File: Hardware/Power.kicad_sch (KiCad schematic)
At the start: 62 parts

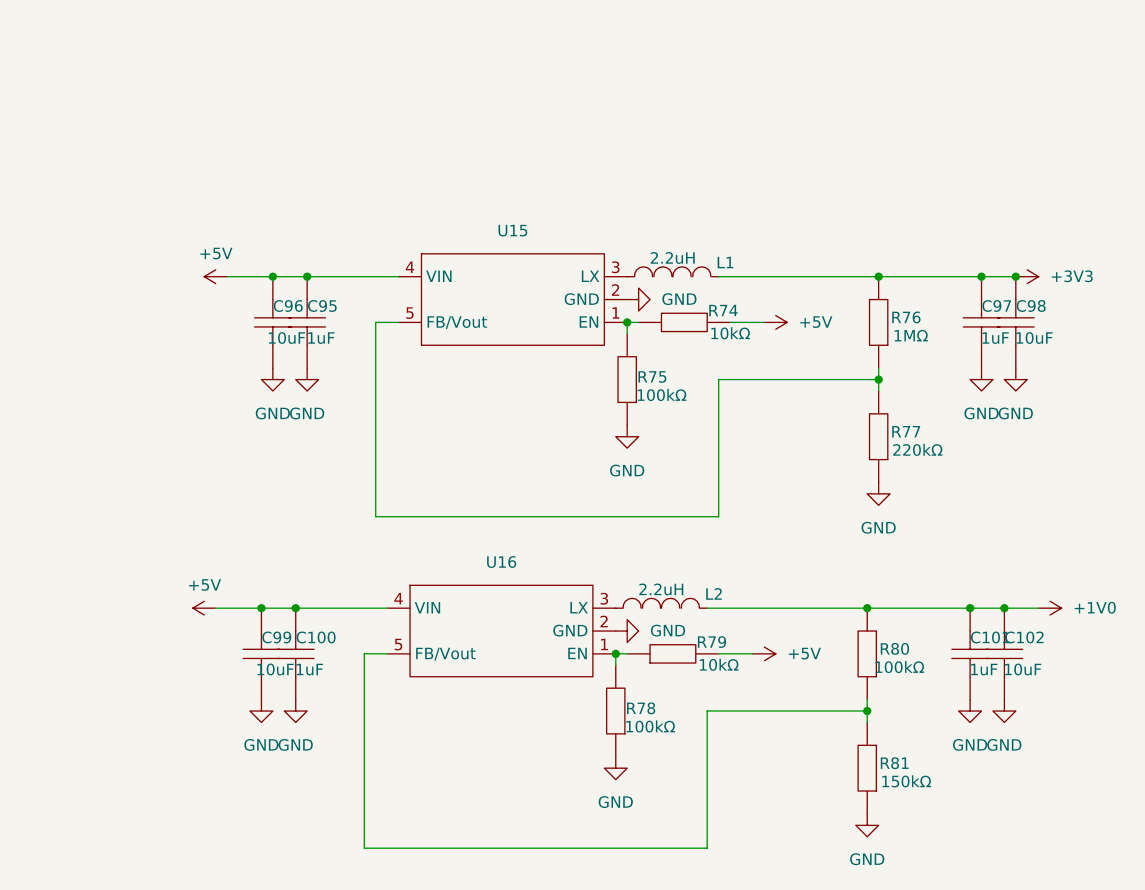
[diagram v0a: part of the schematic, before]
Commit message: 修改了电源供电部分的内容
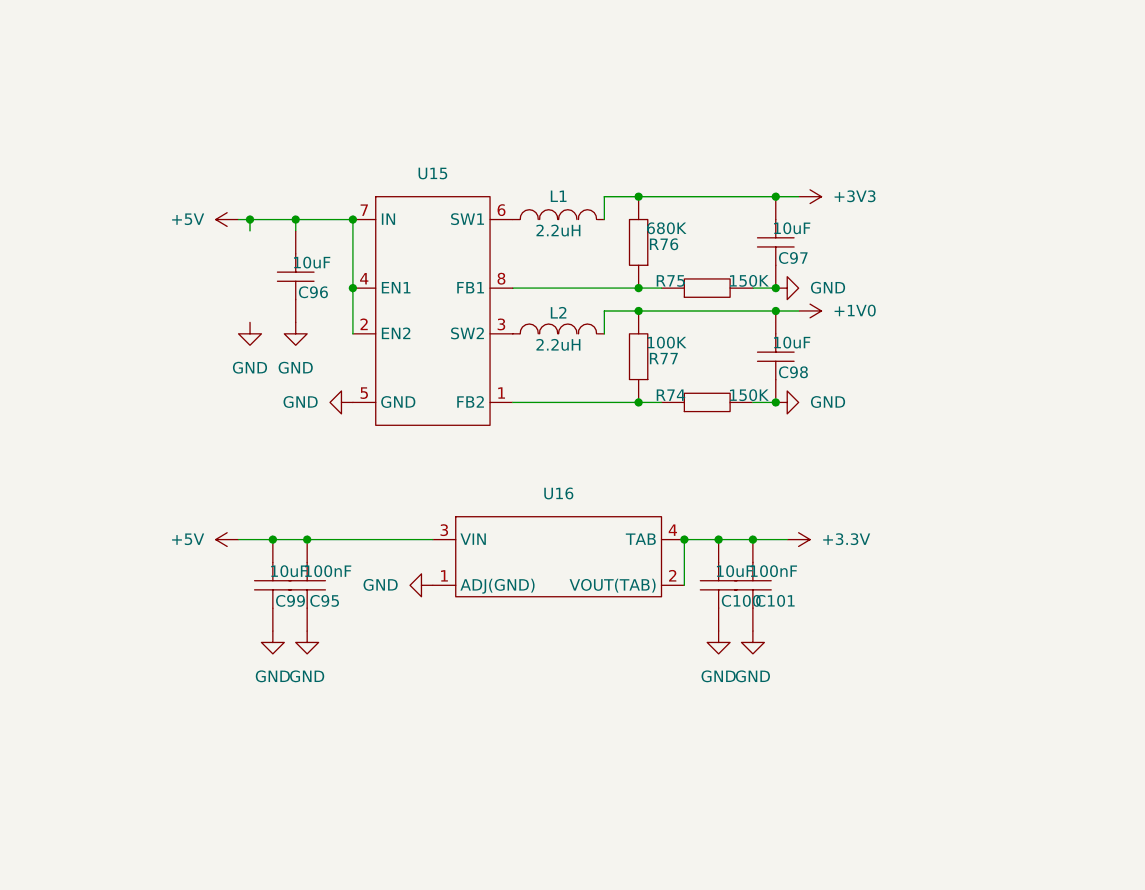
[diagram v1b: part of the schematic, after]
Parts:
- removed C102: 10uF, persional_library:C0603, symbol persional_library:C0603
- removed R78, R80: 100kΩ, persional_library:R0603, symbol persional_library:R0603
- removed R79: 10kΩ, persional_library:R0603, symbol persional_library:R0603
- removed R81: 150kΩ, persional_library:R0603, symbol persional_library:R0603
- removed U15, U16: ~, persional_library:SOT-23-5_L3.0-W1.7-P0.95-LS2.8-BR, symbol persional_library:DCDC-LP3220AB5F
- added U15: ~, persional_library:TSOT-23-8_L2.9-W1.6-P0.65-LS2.8-BL, symbol persional_library:DCDC_MP2122AGJ-Z
- added U16: ~, persional_library:SOT-223-4_L6.5-W3.5-P2.30-LS7.0-BR, symbol persional_library:LDO_AMS1117-3.3
- C100, C97: value 1uF -> 10uF
- C101, C95: value 1uF -> 100nF
- R74: value 10kΩ -> 150K
- R75: value 100kΩ -> 150K
- R76: value 1MΩ -> 680K
- R77: value 220kΩ -> 100K
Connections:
- net +1V0: now also C98.2, R77.2; no longer C101.2
- net +3V3: no longer C98.2
- net +5V: now also U15.2 (EN2), U15.4 (EN1), U15.7 (IN), U16.3 (VIN); no longer C100.2, R74.2
- net GND: now also R74.2, R75.2, U15.5 (GND), U16.1 (ADJ(GND)); no longer R75.1, R77.1
- net at R76.1: now also R75.1, U15.8 (FB1); no longer R77.2
- net at R74.1: now also R77.1, U15.1 (FB2); no longer R75.2
- net at L1.1: now also U15.6 (SW1)
- net at L2.1: now also U15.3 (SW2)
- new net +3.3V: C100.2, C101.2, U16.2 (VOUT(TAB)), U16.4 (TAB)
